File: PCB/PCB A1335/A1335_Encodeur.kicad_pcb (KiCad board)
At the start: 2 copper layers, 13 parts, among them P1 CONN_01X04, Q1 MOS_N, Q2 MOS_N, U1 662K, U2 A1335LLETR-T

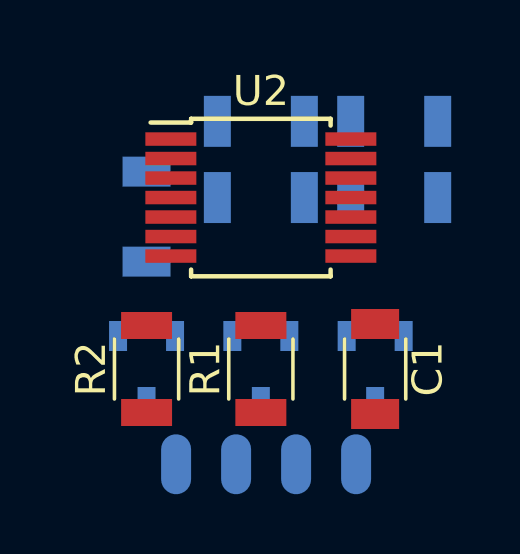
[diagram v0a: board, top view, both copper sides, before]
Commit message: A1335_upload_files
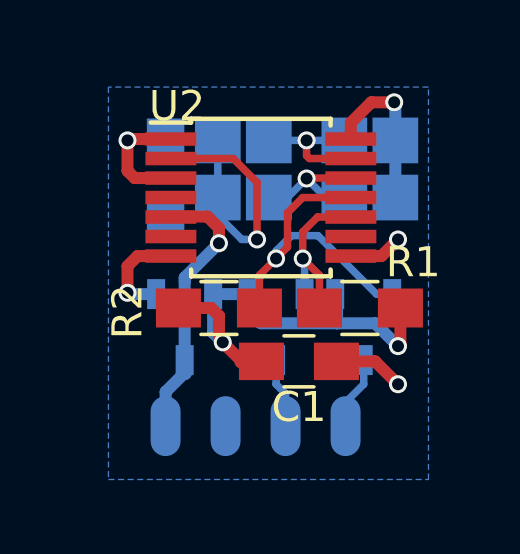
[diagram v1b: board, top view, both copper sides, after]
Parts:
- removed R3, R4, R5, R6: 0, R_1206
- added W1: 0, TESTPT, B.Cu at (129.4, 105.4)
- added W2: 0, TESTPT, B.Cu at (125.1, 105.4)
- added W3: 0, TESTPT, B.Cu at (129.4, 107.3)
- added W4: 0, TESTPT, B.Cu at (125.1, 107.3)
- C1, C2: footprint C_1206 -> C_0805_HandSoldering
- Q1, Q2: value MOS_N -> BSS138
- R1, R2: footprint R_1206 -> R_0805_HandSoldering
- moved Q2 7.37 mm to (129.2, 111.6)
- moved U1 6.50 mm to (123.2, 111.6)
- moved P1 6.48 mm to (122.6, 114.9), turned to 270 degrees
- moved R1 3.88 mm to (129.0, 111.0), turned to 0 degrees
- moved R2 3.15 mm to (124.3, 111.0), turned to 180 degrees
- moved C1 2.55 mm to (127.0, 112.8), turned to 0 degrees
- moved Q1 1.49 mm to (126.2, 111.6)
- moved C2 1.42 mm to (122.6, 106.7), turned to 90 degrees
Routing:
- net GND: track 0.00 -> 18.6 mm, vias 0 -> 5
- net +3.3V: track 0.00 -> 15.2 mm, vias 0 -> 2
- net Net-(C2-Pad1): track 0.00 -> 11.2 mm, vias 0 -> 1
- net /SCL_33: track 0.00 -> 11.0 mm, vias 0 -> 1
- net +5V: track 0.00 -> 9.11 mm, vias 0 -> 1
- net /SDA_33: track 0.00 -> 5.79 mm, vias 0 -> 1
- net Net-(U2-Pad13): track 0.00 -> 4.54 mm, vias 0 -> 1
- net Net-(U2-Pad12): track 0.00 -> 4.53 mm, vias 0 -> 1
- net /SCL: track 0.00 -> 2.45 mm
- net /SDA: track 0.00 -> 2.33 mm
- added copper zone on B.Cu, net GND
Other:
- net class ALIM added: clearance 0.2, trace_width 0.4, via_dia 0.6, via_drill 0.4
